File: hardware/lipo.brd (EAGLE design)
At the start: 33.5 x 34.6 mm, 62 parts, among them IC1 4066D, IC2 4066D, J1 MICRO_USB_B_HIROSE_ZX62-B-5PA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, Q1 IRLML6402, SW1 TVAF06-A020B-R, U1 LT6106CS5#PBF, U2 NJM12888F, U3 MCP73831, U5 TCK106AF,LF, X1 FA-238

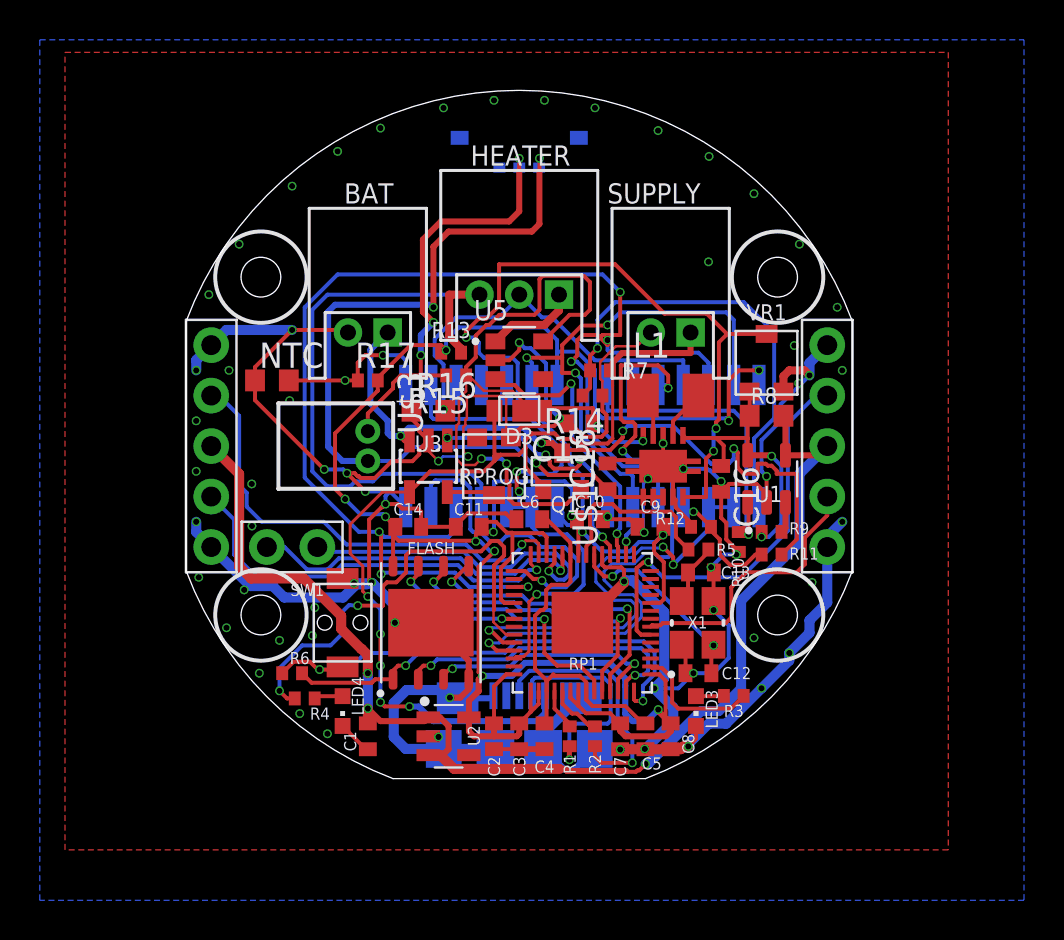
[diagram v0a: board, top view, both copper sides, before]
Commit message: ベタ・シルク調整
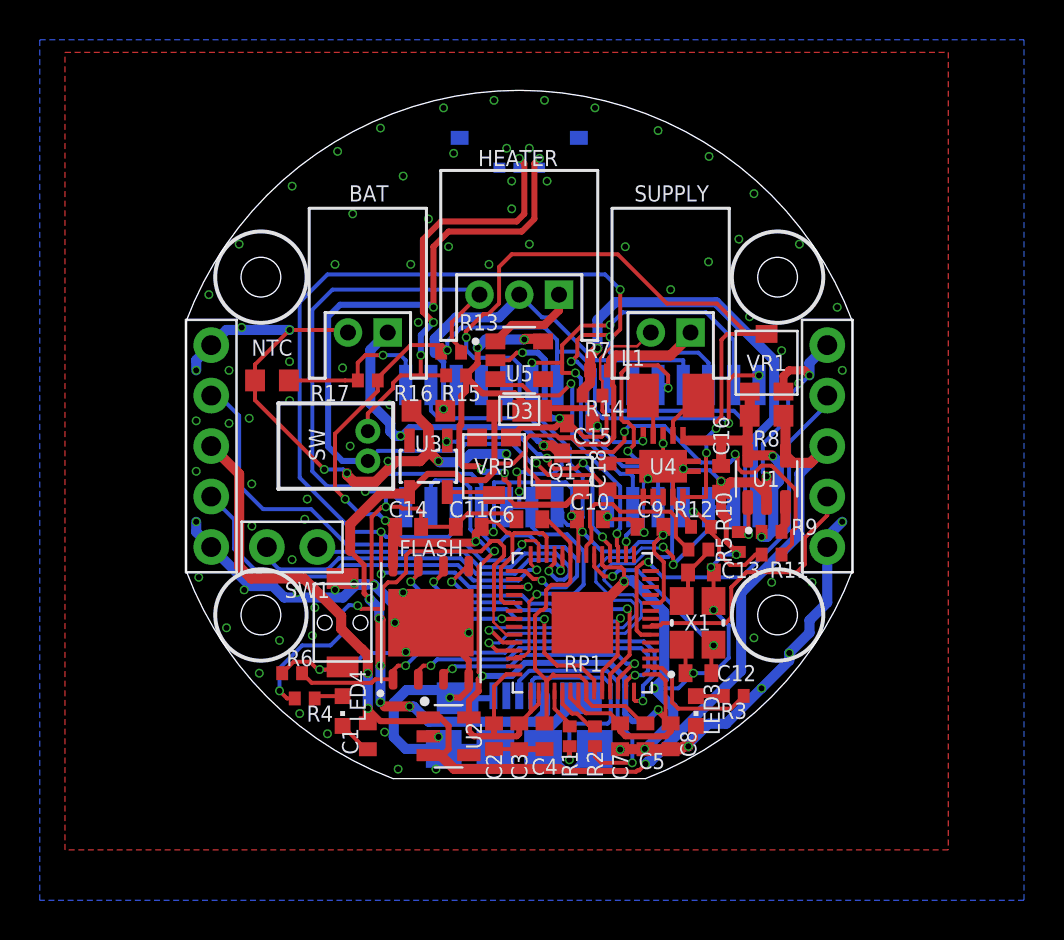
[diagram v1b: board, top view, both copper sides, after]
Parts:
- renumbered RPROG to VRP, U$1 to U4, U$3 to SW
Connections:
- net N$13 renamed HEATER_OUT
- net N$3 renamed VBAT_
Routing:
- net VBAT_: track 39.0 -> 28.9 mm, vias 4 -> 6
- net GND: track 216.9 -> 212.2 mm, vias 71 -> 110
- net VBAT: track 36.0 -> 34.3 mm
- net V+_V: track 44.1 -> 45.5 mm
- net ADC_SEL1: track 28.9 -> 27.7 mm
- net ADC1_IN: track 34.2 -> 33.3 mm
- net SUPPLY_V: track 23.3 -> 22.5 mm
- net TEMP: track 32.0 -> 31.2 mm
- net OB_TEMP: vias 2 -> 1
